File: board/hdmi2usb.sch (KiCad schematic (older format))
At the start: 0 parts

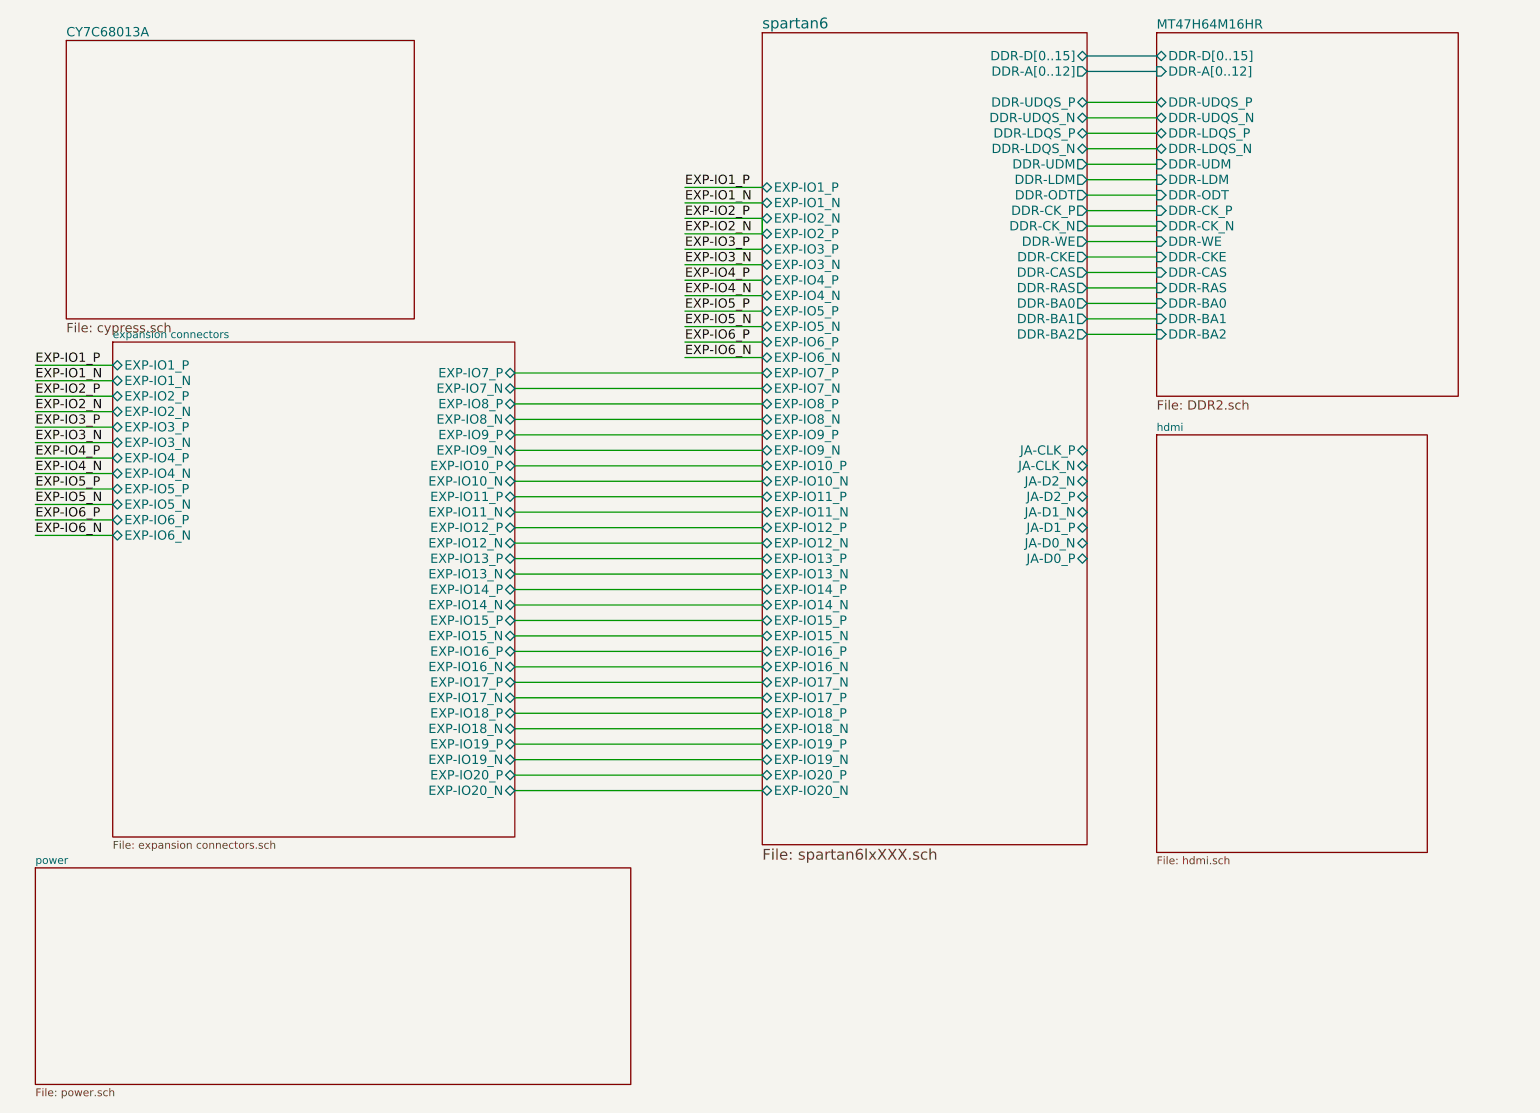
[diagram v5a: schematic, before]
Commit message: Issue #336
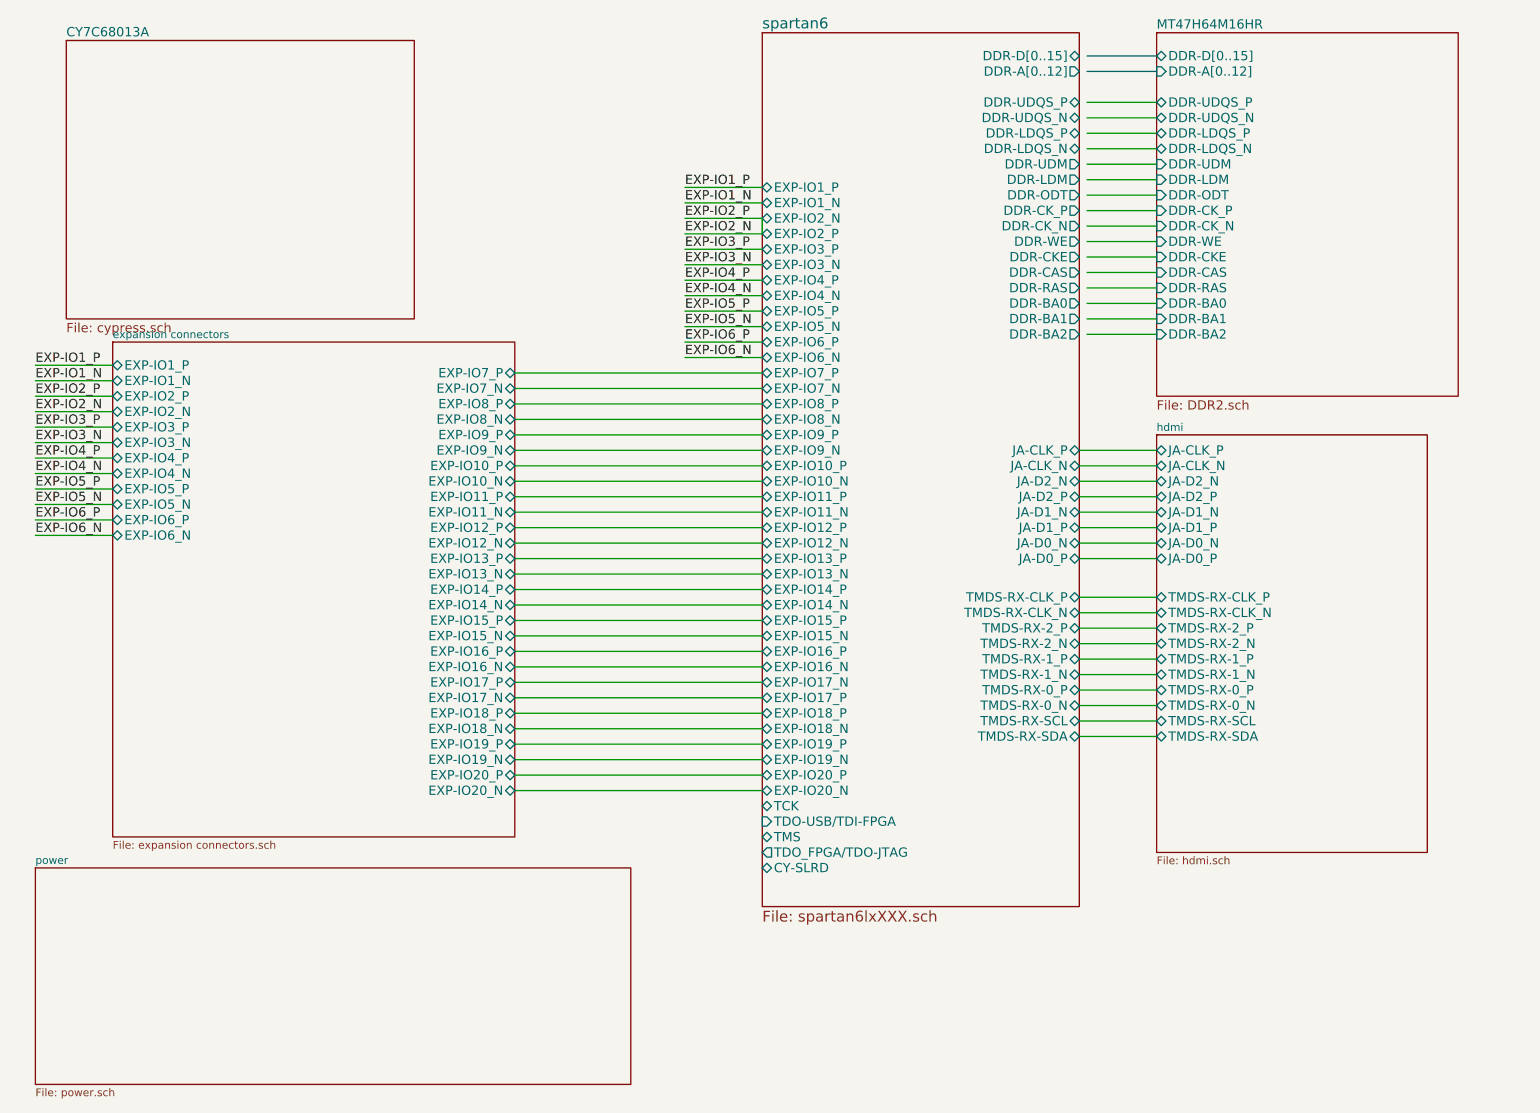
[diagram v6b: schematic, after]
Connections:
- wire segments 69 -> 87
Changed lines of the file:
@@
 F0 "hdmi" 50
 F1 "hdmi.sch" 50
+F2 "TMDS-RX-2_P" B L 8400 4550 60
+F3 "TMDS-RX-1_P" B L 8400 4750 60
+F4 "TMDS-RX-0_P" B L 8400 4950 60
+F5 "TMDS-RX-2_N" B L 8400 4650 60
+F6 "TMDS-RX-1_N" B L 8400 4850 60
+F7 "TMDS-RX-0_N" B L 8400 5050 60
+F8 "TMDS-RX-CLK_P" B L 8400 4350 60
+F9 "TMDS-RX-CLK_N" B L 8400 4450 60
+F10 "TMDS-RX-SCL" B L 8400 5150 60
+F11 "TMDS-RX-SDA" B L 8400 5250 60
+F12 "JA-D2_P" B L 8400 3700 60
+F13 "JA-D2_N" B L 8400 3600 60
+F14 "JA-D1_P" B L 8400 3900 60
+F15 "JA-D1_N" B L 8400 3800 60
+F16 "JA-D0_P" B L 8400 4100 60
+F17 "JA-D0_N" B L 8400 4000 60
+F18 "JA-CLK_P" B L 8400 3400 60
+F19 "JA-CLK_N" B L 8400 3500 60
 $EndSheet
 Wire Wire Line
@@
 Wire Wire Line
 	5850 1900 5850 2000
-$Sheet
-S 5850 700  2100 5250
-U 51AED6DE
-F0 "spartan6" 70
-F1 "spartan6lxXXX.sch" 70
-F2 "DDR-D[0..15]" B R 7950 850 60
-F3 "DDR-A[0..12]" O R 7950 950 60
-F4 "DDR-LDQS_P" B R 7950 1350 60
-F5 "DDR-LDQS_N" B R 7950 1450 60
-F6 "DDR-UDM" O R 7950 1550 60
-F7 "DDR-LDM" O R 7950 1650 60
-F8 "DDR-UDQS_P" B R 7950 1150 60
-F9 "DDR-UDQS_N" B R 7950 1250 60
-F10 "DDR-RAS" O R 7950 2350 60
-F11 "DDR-CAS" O R 7950 2250 60
-F12 "DDR-ODT" O R 7950 1750 60
-F13 "DDR-CK_P" O R 7950 1850 60
-F14 "DDR-CK_N" O R 7950 1950 60
-F15 "DDR-BA0" O R 7950 2450 60
-F16 "DDR-BA1" O R 7950 2550 60
-F17 "DDR-WE" O R 7950 2050 60
-F18 "DDR-BA2" O R 7950 2650 60
-F19 "DDR-CKE" O R 7950 2150 60
-F20 "EXP-IO1_N" B L 5850 1800 60
-F21 "EXP-IO1_P" B L 5850 1700 60
-F22 "EXP-IO10_N" B L 5850 3600 60
-F23 "EXP-IO10_P" B L 5850 3500 60
-F24 "EXP-IO11_P" B L 5850 3700 60
-F25 "EXP-IO11_N" B L 5850 3800 60
-F26 "EXP-IO12_N" B L 5850 4000 60
-F27 "EXP-IO12_P" B L 5850 3900 60
-F28 "JA-CLK_P" B R 7950 3400 60
-F29 "JA-CLK_N" B R 7950 3500 60
-F30 "EXP-IO13_P" B L 5850 4100 60
-F31 "EXP-IO13_N" B L 5850 4200 60
-F32 "EXP-IO14_P" B L 5850 4300 60
-F33 "EXP-IO14_N" B L 5850 4400 60
-F34 "JA-D2_N" B R 7950 3600 60
-F35 "JA-D2_P" B R 7950 3700 60
-F36 "JA-D1_N" B R 7950 3800 60
-F37 "JA-D1_P" B R 7950 3900 60
-F38 "JA-D0_N" B R 7950 4000 60
-F39 "JA-D0_P" B R 7950 4100 60
-F40 "EXP-IO15_P" B L 5850 4500 60
-F41 "EXP-IO15_N" B L 5850 4600 60
-F42 "EXP-IO16_P" B L 5850 4700 60
-F43 "EXP-IO16_N" B L 5850 4800 60
-F44 "EXP-IO17_N" B L 5850 4900 60
-F45 "EXP-IO17_P" B L 5850 5000 60
-F46 "EXP-IO18_P" B L 5850 5100 60
-F47 "EXP-IO18_N" B L 5850 5200 60
-F48 "EXP-IO19_P" B L 5850 5300 60
-F49 "EXP-IO19_N" B L 5850 5400 60
-F50 "EXP-IO2_P" B L 5850 2000 60
-F51 "EXP-IO2_N" B L 5850 1900 60
-F52 "EXP-IO20_N" B L 5850 5600 60
-F53 "EXP-IO20_P" B L 5850 5500 60
-F54 "EXP-IO3_N" B L 5850 2200 60
-F55 "EXP-IO3_P" B L 5850 2100 60
-F56 "EXP-IO4_N" B L 5850 2400 60
-F57 "EXP-IO4_P" B L 5850 2300 60
-F58 "EXP-IO5_N" B L 5850 2600 60
-F59 "EXP-IO5_P" B L 5850 2500 60
-F60 "EXP-IO6_N" B L 5850 2800 60
-F61 "EXP-IO6_P" B L 5850 2700 60
-F62 "EXP-IO7_N" B L 5850 3000 60
-F63 "EXP-IO7_P" B L 5850 2900 60
-F64 "EXP-IO8_N" B L 5850 3200 60
-F65 "EXP-IO8_P" B L 5850 3100 60
-F66 "EXP-IO9_N" B L 5850 3400 60
-F67 "EXP-IO9_P" B L 5850 3300 60
-$EndSheet
 Wire Wire Line
 	5850 2900 4250 2900
@@
 Wire Wire Line
 	5850 5600 4250 5600
+$Sheet
+S 5850 700  2050 5650
+U 51AED6DE
+F0 "spartan6" 70
+F1 "spartan6lxXXX.sch" 70
+F2 "DDR-D[0..15]" B R 7900 850 60
+F3 "DDR-A[0..12]" O R 7900 950 60
+F4 "DDR-LDQS_P" B R 7900 1350 60
+F5 "DDR-LDQS_N" B R 7900 1450 60
+F6 "DDR-UDM" O R 7900 1550 60
+F7 "DDR-LDM" O R 7900 1650 60
+F8 "DDR-UDQS_P" B R 7900 1150 60
+F9 "DDR-UDQS_N" B R 7900 1250 60
+F10 "DDR-RAS" O R 7900 2350 60
+F11 "DDR-CAS" O R 7900 2250 60
+F12 "DDR-ODT" O R 7900 1750 60
+F13 "DDR-CK_P" O R 7900 1850 60
+F14 "DDR-CK_N" O R 7900 1950 60
+F15 "DDR-BA0" O R 7900 2450 60
+F16 "DDR-BA1" O R 7900 2550 60
+F17 "DDR-WE" O R 7900 2050 60
+F18 "DDR-BA2" O R 7900 2650 60
+F19 "DDR-CKE" O R 7900 2150 60
+F20 "EXP-IO1_N" B L 5850 1800 60
+F21 "EXP-IO1_P" B L 5850 1700 60
+F22 "EXP-IO10_N" B L 5850 3600 60
+F23 "EXP-IO10_P" B L 5850 3500 60
+F24 "EXP-IO11_P" B L 5850 3700 60
+F25 "EXP-IO11_N" B L 5850 3800 60
+F26 "EXP-IO12_N" B L 5850 4000 60
+F27 "EXP-IO12_P" B L 5850 3900 60
+F28 "JA-CLK_P" B R 7900 3400 60
+F29 "JA-CLK_N" B R 7900 3500 60
+F30 "EXP-IO13_P" B L 5850 4100 60
+F31 "EXP-IO13_N" B L 5850 4200 60
+F32 "EXP-IO14_P" B L 5850 4300 60
+F33 "EXP-IO14_N" B L 5850 4400 60
+F34 "JA-D2_N" B R 7900 3600 60
+F35 "JA-D2_P" B R 7900 3700 60
+F36 "JA-D1_N" B R 7900 3800 60
+F37 "JA-D1_P" B R 7900 3900 60
+F38 "JA-D0_N" B R 7900 4000 60
+F39 "JA-D0_P" B R 7900 4100 60
+F40 "EXP-IO15_P" B L 5850 4500 60
+F41 "EXP-IO15_N" B L 5850 4600 60
+F42 "EXP-IO16_P" B L 5850 4700 60
+F43 "EXP-IO16_N" B L 5850 4800 60
+F44 "EXP-IO17_N" B L 5850 4900 60
+F45 "EXP-IO17_P" B L 5850 5000 60
+F46 "EXP-IO18_P" B L 5850 5100 60
+F47 "EXP-IO18_N" B L 5850 5200 60
+F48 "EXP-IO19_P" B L 5850 5300 60
+F49 "EXP-IO19_N" B L 5850 5400 60
+F50 "EXP-IO2_P" B L 5850 2000 60
+F51 "EXP-IO2_N" B L 5850 1900 60
+F52 "EXP-IO20_N" B L 5850 5600 60
+F53 "EXP-IO20_P" B L 5850 5500 60
+F54 "EXP-IO3_N" B L 5850 2200 60
+F55 "EXP-IO3_P" B L 5850 2100 60
+F56 "EXP-IO4_N" B L 5850 2400 60
+F57 "EXP-IO4_P" B L 5850 2300 60
+F58 "EXP-IO5_N" B L 5850 2600 60
+F59 "EXP-IO5_P" B L 5850 2500 60
+F60 "EXP-IO6_N" B L 5850 2800 60
+F61 "EXP-IO6_P" B L 5850 2700 60
+F62 "EXP-IO7_N" B L 5850 3000 60
+F63 "EXP-IO7_P" B L 5850 2900 60
+F64 "EXP-IO8_N" B L 5850 3200 60
+F65 "EXP-IO8_P" B L 5850 3100 60
+F66 "EXP-IO9_N" B L 5850 3400 60
+F67 "EXP-IO9_P" B L 5850 3300 60
+F68 "TMDS-RX-CLK_P" B R 7900 4350 60
+F69 "TMDS-RX-CLK_N" B R 7900 4450 60
+F70 "TMDS-RX-2_P" B R 7900 4550 60
+F71 "TMDS-RX-2_N" B R 7900 4650 60
+F72 "TMDS-RX-0_P" B R 7900 4950 60
+F73 "TMDS-RX-0_N" B R 7900 5050 60
+F74 "TMDS-RX-1_P" B R 7900 4750 60
+F75 "TMDS-RX-1_N" B R 7900 4850 60
+F76 "TMDS-RX-SCL" B R 7900 5150 60
+F77 "TMDS-RX-SDA" B R 7900 5250 60
+F78 "TCK" B L 5850 5700 60
+F79 "TDO-USB/TDI-FPGA" I L 5850 5800 60
+F80 "TMS" B L 5850 5900 60
+F81 "TDO_FPGA/TDO-JTAG" O L 5850 6000 60
+F82 "CY-SLRD" B L 5850 6100 60
+$EndSheet
+Wire Wire Line
+	7900 3400 8400 3400
+Wire Wire Line
+	7900 3500 8400 3500
+Wire Wire Line
+	7900 3600 8400 3600
+Wire Wire Line
+	7900 3700 8400 3700
+Wire Wire Line
+	7900 3800 8400 3800
+Wire Wire Line
+	7900 3900 8400 3900
+Wire Wire Line
+	7900 4000 8400 4000
+Wire Wire Line
+	7900 4100 8400 4100
+Wire Wire Line
+	7900 4350 8400 4350
+Wire Wire Line
+	7900 4450 8400 4450
+Wire Wire Line
+	7900 4550 8400 4550
+Wire Wire Line
+	7900 4650 8400 4650
+Wire Wire Line
+	7900 4750 8400 4750
+Wire Wire Line
+	7900 4850 8400 4850
+Wire Wire Line
+	7900 4950 8400 4950
+Wire Wire Line
+	8400 5050 7900 5050
+Wire Wire Line
+	7900 5150 8400 5150
+Wire Wire Line
+	8400 5250 7900 5250
 $EndSCHEMATC
